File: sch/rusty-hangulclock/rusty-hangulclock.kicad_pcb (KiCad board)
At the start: 2 copper layers, 45 x 54 mm, 14 parts, among them J1 Conn_OLED, J2 Conn_SLEDS, J3 PWR, SW1 RotaryEncoder_Switch_MP

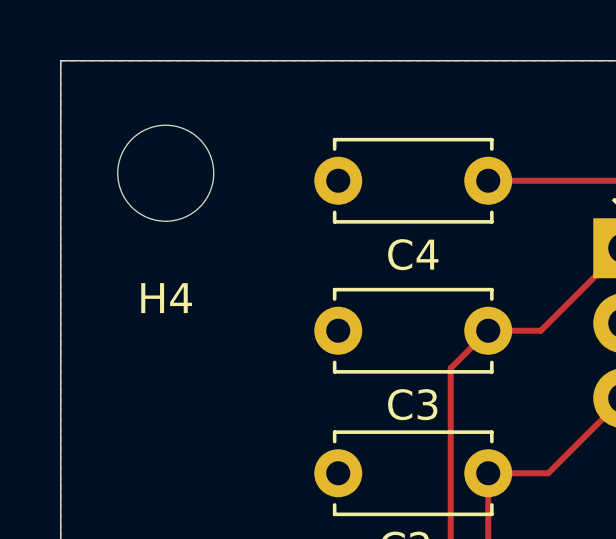
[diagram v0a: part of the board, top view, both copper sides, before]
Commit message: sch: fix pcb
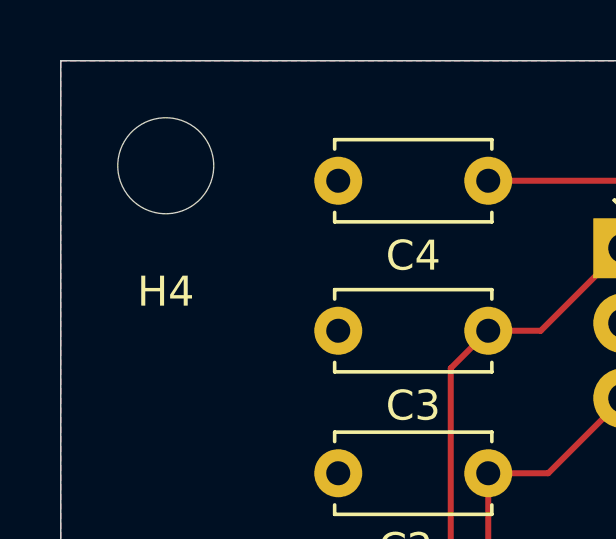
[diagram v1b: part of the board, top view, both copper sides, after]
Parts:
- moved H4 0.25 mm to (124.5, 88.5)
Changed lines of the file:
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@@
 		)
 		(fp_text user "${REFERENCE}"
-			(at 0 1.27 360)
+			(at 0 1.27 0)
 			(layer "F.Fab")
 			(effects
@@
 		(tags "C Disc series Radial pin pitch 5.00mm  diameter 5mm width 2.5mm Capacitor")
 		(property "Reference" "C4"
-			(at 2.5 -2.5 360)
+			(at 2.5 -2.5 0)
 			(layer "F.SilkS")
 			(effects
@@
 		)
 		(property "Value" "100n"
-			(at 2.5 2.5 360)
+			(at 2.5 2.5 0)
 			(layer "F.Fab")
 			(effects
@@
 		)
 		(fp_text user "${REFERENCE}"
-			(at 2.5 0 360)
+			(at 2.5 0 0)
 			(layer "F.Fab")
 			(effects
@@
 		(tags "rotary encoder")
 		(property "Reference" "SW1"
-			(at 2.8 -4.7 360)
+			(at 2.8 -4.7 0)
 			(layer "F.SilkS")
 			(effects
@@
 		)
 		(property "Value" "RotaryEncoder_Switch_MP"
-			(at 7.5 10.4 360)
+			(at 7.5 10.4 0)
 			(layer "F.Fab")
 			(effects
@@
 		)
 		(fp_text user "${REFERENCE}"
-			(at 11.1 6.3 360)
+			(at 11.1 6.3 0)
 			(layer "F.Fab")
 			(effects
@@
 		(tags "C Disc series Radial pin pitch 5.00mm  diameter 5mm width 2.5mm Capacitor")
 		(property "Reference" "C2"
-			(at 2.75 -2.5 360)
+			(at 2.75 -2.5 0)
 			(layer "F.SilkS")
 			(effects
@@
 		)
 		(property "Value" "100n"
-			(at 2.5 2.5 360)
+			(at 2.5 2.5 0)
 			(layer "F.Fab")
 			(effects
@@
 		)
 		(fp_text user "${REFERENCE}"
-			(at 2.5 0 360)
+			(at 2.5 0 0)
 			(layer "F.Fab")
 			(effects
@@
 		(tags "Through hole angled pin header THT 1x04 2.54mm single row")
 		(property "Reference" "J2"
-			(at 4.385 -2.27 360)
+			(at 4.385 -2.27 0)
 			(layer "F.SilkS")
 			(effects
@@
 		)
 		(property "Value" "Conn_SLEDS"
-			(at 4.385 9.89 360)
+			(at 4.385 9.89 0)
 			(layer "F.Fab")
 			(effects
@@
 	(footprint "MountingHole:MountingHole_3.2mm_M3"
 		(layer "F.Cu")
-		(at 124.5 88.75 180)
+		(at 124.5 88.5 180)
 		(descr "Mounting Hole 3.2mm, no annular, M3")
 		(tags "mounting hole 3.2mm no annular m3")
@@
 		(tags "CP Radial series Radial pin pitch 2.00mm  diameter 4mm Electrolytic Capacitor")
 		(property "Reference" "C1"
-			(at 1 -3.25 360)
+			(at 1 -3.25 0)
 			(layer "F.SilkS")
 			(effects
@@
 		)
 		(property "Value" "C_Polarized"
-			(at 1 3.25 360)
+			(at 1 3.25 0)
 			(layer "F.Fab")
 			(effects
@@
 		)
 		(fp_text user "${REFERENCE}"
-			(at 1 0 360)
+			(at 1 0 0)
 			(layer "F.Fab")
 			(effects
@@
 		(at 127.75 123.75)
 		(property "Reference" "G***"
-			(at 0 0 360)
+			(at 0 0 0)
 			(layer "F.SilkS")
 			(hide yes)
@@
 		)
 		(property "Value" "LOGO"
-			(at 0.75 0 360)
+			(at 0.75 0 0)
 			(layer "F.SilkS")
 			(hide yes)
@@
 		)
 		(property "Footprint" ""
-			(at 0 0 360)
+			(at 0 0 0)
 			(layer "F.Fab")
 			(hide yes)
@@
 		)
 		(property "Datasheet" ""
-			(at 0 0 360)
+			(at 0 0 0)
 			(layer "F.Fab")
 			(hide yes)
@@
 		)
 		(property "Description" ""
-			(at 0 0 360)
+			(at 0 0 0)
 			(layer "F.Fab")
 			(hide yes)
@@
 		(tags "C Disc series Radial pin pitch 5.00mm  diameter 5mm width 2.5mm Capacitor")
 		(property "Reference" "C3"
-			(at 2.5 -2.5 360)
+			(at 2.5 -2.5 0)
 			(layer "F.SilkS")
 			(effects
@@
 		)
 		(property "Value" "100n"
-			(at 2.5 2.5 360)
+			(at 2.5 2.5 0)
 			(layer "F.Fab")
 			(effects
@@
 		)
 		(fp_text user "${REFERENCE}"
-			(at 2.5 0 360)
+			(at 2.5 0 0)
 			(layer "F.Fab")
 			(effects
